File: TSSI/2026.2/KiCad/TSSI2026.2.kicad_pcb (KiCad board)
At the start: 2 copper layers, 66 x 35 mm, 32 parts, among them J1 Conn_01x02, J2 Conn_01x02, J3 Conn_02x02, Q1 IRLZ34N, T555 Test555, U1 LM555xN, U2 IRLZ34N, U3 IRLZ34N, U4 4001, U5 4069

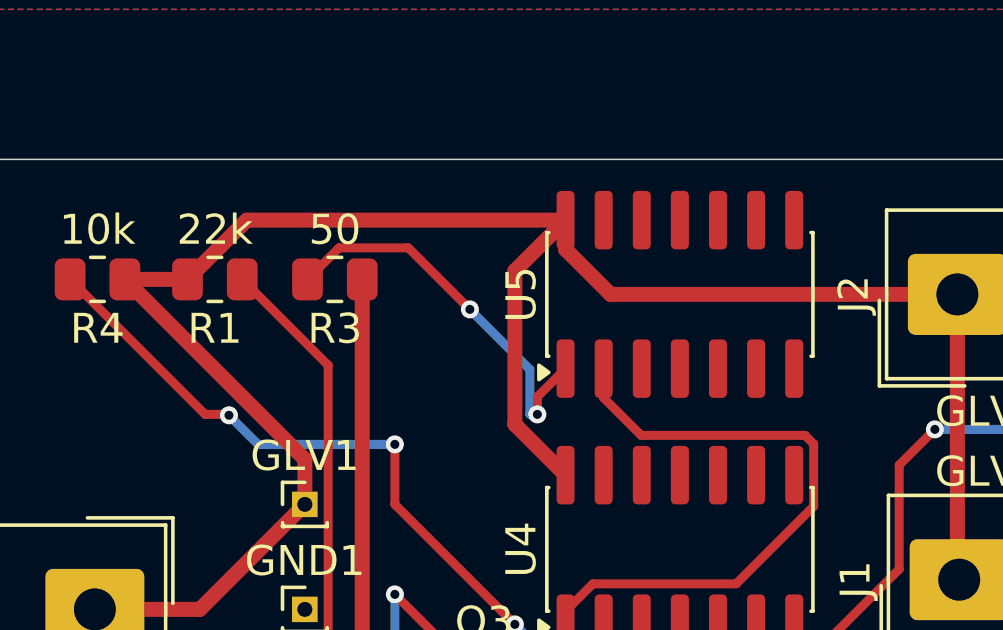
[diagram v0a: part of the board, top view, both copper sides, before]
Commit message: Add files via upload
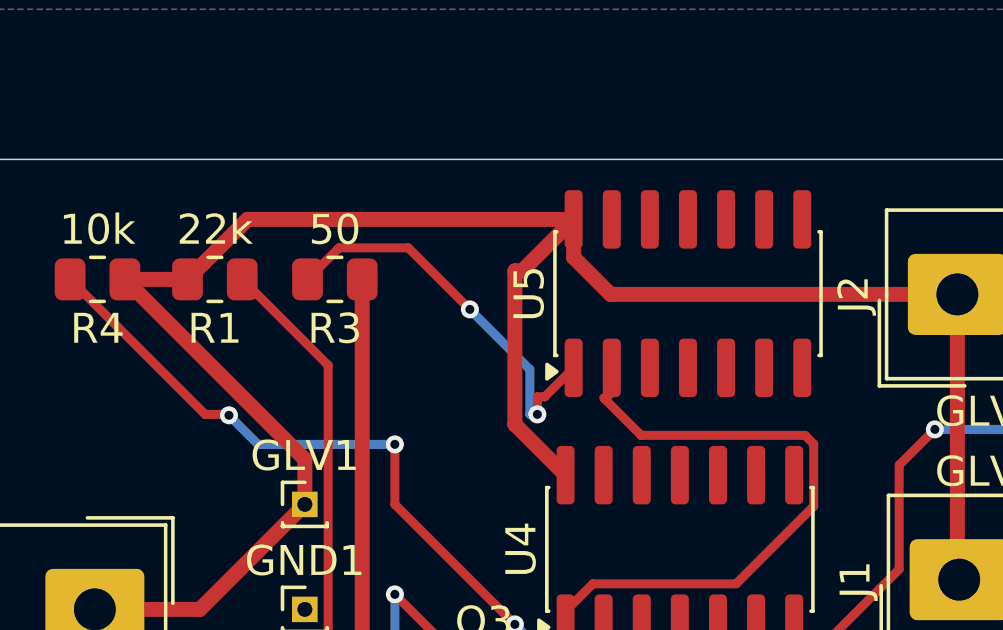
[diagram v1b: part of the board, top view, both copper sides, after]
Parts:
- moved U5 0.27 mm to (72.3, 24.5)
